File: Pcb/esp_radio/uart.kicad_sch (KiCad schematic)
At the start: 12 parts, among them J12 USB_B_Micro, Q1 SS8050G, Q2 SS8050G, U6 CH340C

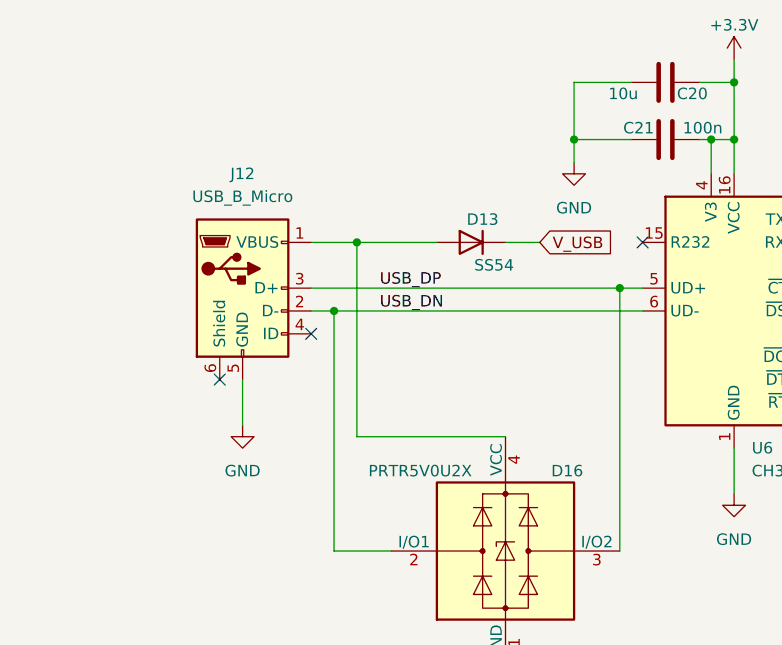
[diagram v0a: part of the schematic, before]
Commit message: Finish board routing
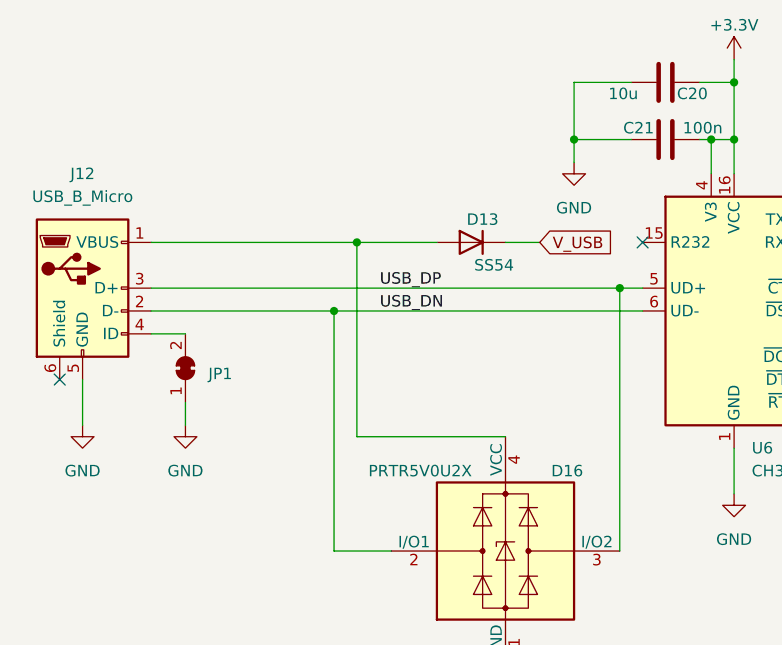
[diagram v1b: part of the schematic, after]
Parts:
- added JP1: SolderJumper_2_Bridged, Jumper:SolderJumper-2_P1.3mm_Bridged_RoundedPad1.0x1.5mm, symbol Jumper:SolderJumper_2_Bridged
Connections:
- net GND: now also JP1.1 (A)
- net at J12.4 (ID): now also JP1.2 (B)
- no-connect marks 7 -> 6
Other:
- moved on the sheet: J12
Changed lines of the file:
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@@
   )
   (no_connect (at 132.08 90.17))
-  (no_connect (at 64.77 92.71))
-  (no_connect (at 74.93 87.63))
+  (no_connect (at 46.99 92.71))
   (no_connect (at 132.08 85.09))
   (no_connect (at 111.76 77.47))
@@
     (stroke (width 0) (type solid))
   )
+  (wire (pts (xy 57.15 87.63) (xy 60.96 87.63))
+    (stroke (width 0) (type default))
+  )
   (wire (pts (xy 119.38 66.04) (xy 121.92 66.04))
     (stroke (width 0) (type solid))
@@
     (stroke (width 0) (type default))
   )
-  (wire (pts (xy 74.93 85.09) (xy 77.47 85.09))
+  (wire (pts (xy 57.15 85.09) (xy 77.47 85.09))
     (stroke (width 0) (type solid))
   )
@@
     (stroke (width 0) (type default))
   )
+  (wire (pts (xy 60.96 95.25) (xy 60.96 97.79))
+    (stroke (width 0) (type default))
+  )
   (wire (pts (xy 118.11 59.69) (xy 121.92 59.69))
     (stroke (width 0) (type solid))
@@
     (stroke (width 0) (type default))
   )
+  (wire (pts (xy 77.47 85.09) (xy 77.47 111.76))
+    (stroke (width 0) (type solid))
+  )
   (wire (pts (xy 96.52 77.47) (xy 100.33 77.47))
     (stroke (width 0) (type solid))
@@
     (stroke (width 0) (type default))
   )
-  (wire (pts (xy 67.31 92.71) (xy 67.31 97.79))
+  (wire (pts (xy 49.53 92.71) (xy 49.53 97.79))
     (stroke (width 0) (type solid))
   )
@@
     (stroke (width 0) (type default))
   )
-  (wire (pts (xy 74.93 77.47) (xy 80.01 77.47))
+  (wire (pts (xy 57.15 77.47) (xy 80.01 77.47))
     (stroke (width 0) (type solid))
   )
@@
     (stroke (width 0) (type default))
   )
-  (wire (pts (xy 77.47 85.09) (xy 77.47 111.76))
-    (stroke (width 0) (type solid))
-  )
   (wire (pts (xy 96.52 99.06) (xy 80.01 99.06))
     (stroke (width 0) (type solid))
@@
     (stroke (width 0) (type solid))
   )
-  (wire (pts (xy 74.93 82.55) (xy 109.22 82.55))
+  (wire (pts (xy 57.15 82.55) (xy 109.22 82.55))
     (stroke (width 0) (type solid))
   )
@@
     )
   )
-  (symbol (lib_id "power:GND") (at 67.31 97.79 0) (unit 1)
-    (in_bom yes) (on_board yes) (dnp no) (fields_autoplaced)
-    (property "Reference" "#PWR040" (at 67.31 104.14 0)
-      (effects (font (size 1.27 1.27)) hide)
-    )
-    (property "Value" "GND" (at 67.31 102.87 0)
-      (effects (font (size 1.27 1.27)))
-    )
-    (property "Footprint" "" (at 67.31 97.79 0)
-      (effects (font (size 1.27 1.27)) hide)
-    )
-    (property "Datasheet" "" (at 67.31 97.79 0)
+  (symbol (lib_id "power:GND") (at 60.96 97.79 0) (unit 1)
+    (in_bom yes) (on_board yes) (dnp no) (fields_autoplaced)
+    (property "Reference" "#PWR072" (at 60.96 104.14 0)
+      (effects (font (size 1.27 1.27)) hide)
+    )
+    (property "Value" "GND" (at 60.96 102.87 0)
+      (effects (font (size 1.27 1.27)))
+    )
+    (property "Footprint" "" (at 60.96 97.79 0)
+      (effects (font (size 1.27 1.27)) hide)
+    )
+    (property "Datasheet" "" (at 60.96 97.79 0)
+      (effects (font (size 1.27 1.27)) hide)
+    )
+    (pin "1")
+    (instances
+      (project "esp_radio"
+        (path "/c9e2e0d2-0655-4f5e-8e13-71b41b1f7cfe/9103cc11-86bf-4fa8-956b-660d9ba42360"
+          (reference "#PWR072") (unit 1)
+        )
+      )
+    )
+  )
+  (symbol (lib_id "power:GND") (at 49.53 97.79 0) (unit 1)
+    (in_bom yes) (on_board yes) (dnp no) (fields_autoplaced)
+    (property "Reference" "#PWR040" (at 49.53 104.14 0)
+      (effects (font (size 1.27 1.27)) hide)
+    )
+    (property "Value" "GND" (at 49.53 102.87 0)
+      (effects (font (size 1.27 1.27)))
+    )
+    (property "Footprint" "" (at 49.53 97.79 0)
+      (effects (font (size 1.27 1.27)) hide)
+    )
+    (property "Datasheet" "" (at 49.53 97.79 0)
       (effects (font (size 1.27 1.27)) hide)
     )
@@
     )
   )
-  (symbol (lib_id "Connector:USB_B_Micro") (at 67.31 82.55 0) (unit 1)
-    (in_bom yes) (on_board yes) (dnp no)
-    (property "Reference" "J12" (at 67.31 69.85 0)
-      (effects (font (size 1.27 1.27)))
-    )
-    (property "Value" "USB_B_Micro" (at 67.31 72.39 0)
-      (effects (font (size 1.27 1.27)))
-    )
-    (property "Footprint" "Connector_PinHeader_2.54mm:PinHeader_1x05_P2.54mm_Vertical" (at 71.12 83.82 0)
-      (effects (font (size 1.27 1.27)) hide)
-    )
-    (property "Datasheet" "~" (at 71.12 83.82 0)
-      (effects (font (size 1.27 1.27)) hide)
-    )
+  (symbol (lib_id "Jumper:SolderJumper_2_Bridged") (at 60.96 91.44 90) (unit 1)
+    (in_bom yes) (on_board yes) (dnp no) (fields_autoplaced)
+    (property "Reference" "JP1" (at 63.5 92.075 90)
+      (effects (font (size 1.27 1.27)) (justify right))
+    )
+    (property "Value" "SolderJumper_2_Bridged" (at 58.42 91.44 0)
+      (effects (font (size 1.27 1.27)) hide)
+    )
+    (property "Footprint" "Jumper:SolderJumper-2_P1.3mm_Bridged_RoundedPad1.0x1.5mm" (at 60.96 91.44 0)
+      (effects (font (size 1.27 1.27)) hide)
+    )
+    (property "Datasheet" "~" (at 60.96 91.44 0)
+      (effects (font (size 1.27 1.27)) hide)
+    )
+    (pin "1")
+    (pin "2")
+    (instances
+      (project "esp_radio"
+        (path "/c9e2e0d2-0655-4f5e-8e13-71b41b1f7cfe/9686c251-96de-4991-9702-894d5bd1468a"
+          (reference "JP1") (unit 1)
+        )
+        (path "/c9e2e0d2-0655-4f5e-8e13-71b41b1f7cfe/9103cc11-86bf-4fa8-956b-660d9ba42360"
+          (reference "JP5") (unit 1)
+        )
+      )
+    )
+  )
+  (symbol (lib_id "Connector:USB_B_Micro") (at 49.53 82.55 0) (unit 1)
+    (in_bom yes) (on_board yes) (dnp no)
+    (property "Reference" "J12" (at 49.53 69.85 0)
+      (effects (font (size 1.27 1.27)))
+    )
+    (property "Value" "USB_B_Micro" (at 49.53 72.39 0)
+      (effects (font (size 1.27 1.27)))
+    )
+    (property "Footprint" "Connector_PinHeader_2.54mm:PinHeader_1x05_P2.54mm_Vertical" (at 53.34 83.82 0)
+      (effects (font (size 1.27 1.27)) hide)
+    )
+    (property "Datasheet" "~" (at 53.34 83.82 0)
+      (effects (font (size 1.27 1.27)) hide)
+    )
